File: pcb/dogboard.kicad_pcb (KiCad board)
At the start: 6 copper layers, 50 x 30 mm, 55 parts, among them J1 USB-C / USB2.0, J2 Lights, J3 Current Conn, SW1 BOOT, SW2 Action, SW3 Action, U1 RP2040, U2 L9110H, U3 4MB Flash, U4 BCR430, Y1 12 MHz

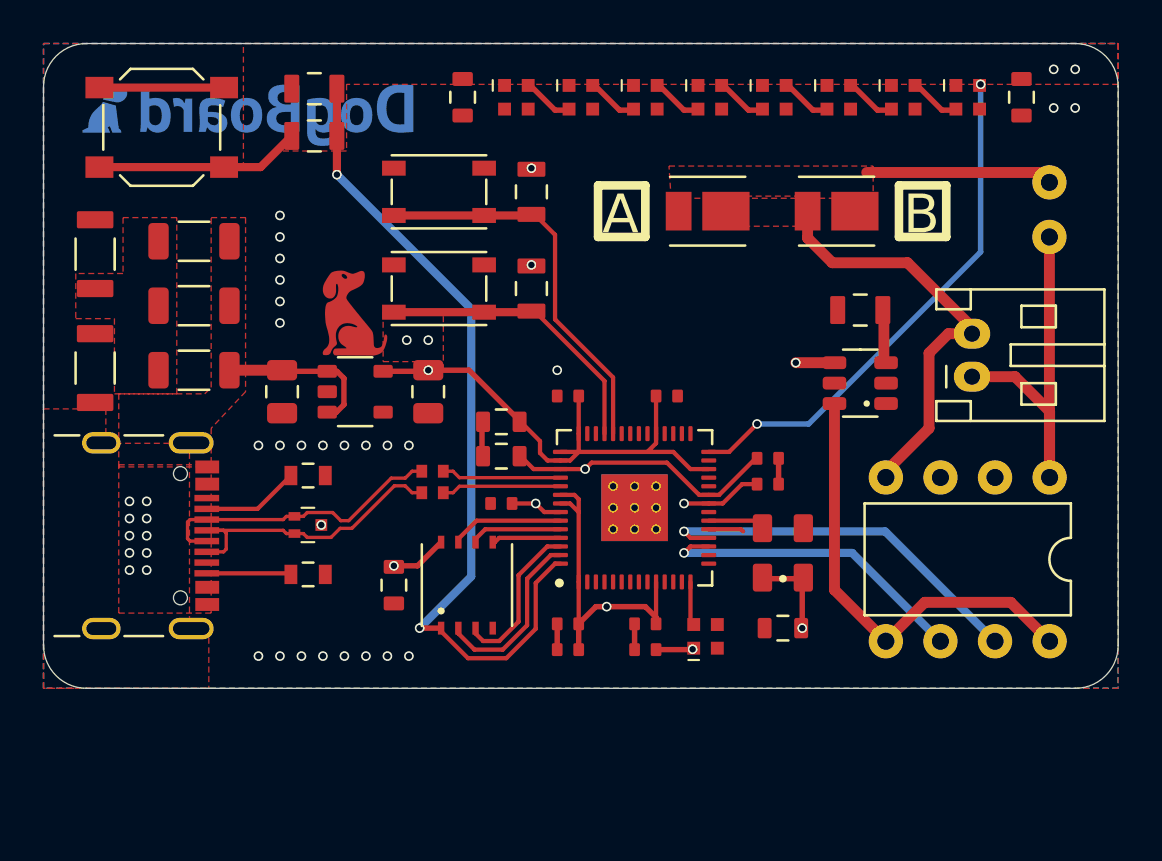
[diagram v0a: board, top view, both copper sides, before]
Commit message: dogboard-2b3
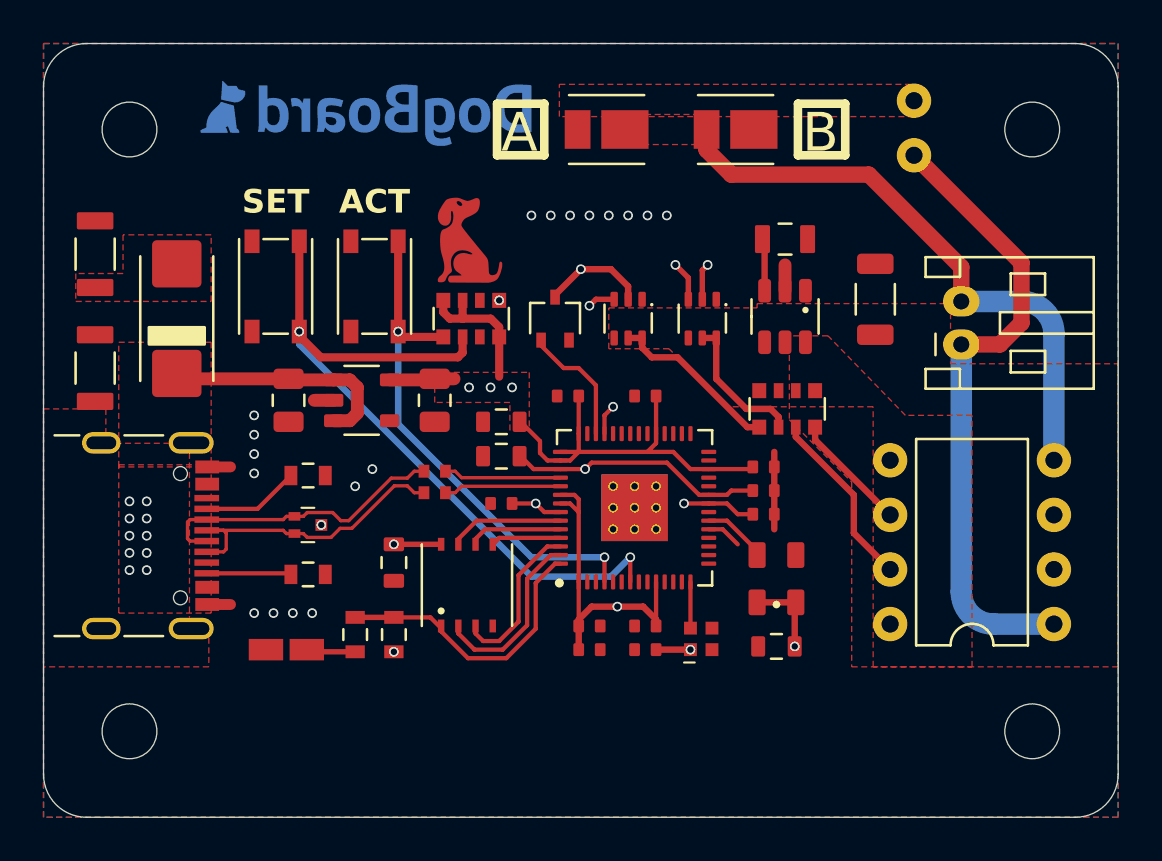
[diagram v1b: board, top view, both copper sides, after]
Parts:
- removed C19, C20: 1uF, _custom:CAP_0603_HandSolder
- removed D10, D2, D3, D4, D5, D7, D8, D9: LED_NeoPixel, _custom:LED_NeoPixel_0606
- removed R12: 10k, _custom:R_0805_HandSolder
- removed SW1: BOOT, _custom:button_metal_smd
- added H1: MountingHole, _custom:MountingHole_M2.5, F.Cu at (128.0, 88.0)
- added H2: MountingHole, _custom:MountingHole_M2.5, F.Cu at (170.0, 88.0)
- added H3: MountingHole, _custom:MountingHole_M2.5, F.Cu at (170.0, 116.0)
- added H4: MountingHole, _custom:MountingHole_M2.5, F.Cu at (128.0, 116.0)
- added JP1: Boot-Jumper, _custom:Jumper_Open_SMD_3.5mm, F.Cu at (135.3, 112.2)
- added Q1: MOSFET, _custom:GenericIC_SOT-363, F.Cu at (154.7, 96.8)
- added Q2: MOSFET, _custom:GenericIC_SOT-363, F.Cu at (151.2, 96.8)
- added Q3: N-MOS, _custom:Transistor_SOT-323, F.Cu at (147.8, 96.8)
- added R9: 10k, _custom:R_Array_4x1206_Convex, F.Cu at (158.6, 101.0)
- C1: value 10uF -> 150uF; footprint _custom:CAP_1206_NoKeepout -> _custom:CAP_Tantalum_2312
- C2: value 10uF -> 10u
- C3: value 10uF -> 0.1u; footprint _custom:CAP_1206_NoKeepout -> _custom:CAP_0402_HandSolder
- R10: footprint _custom:R_0805_HandSolder -> _custom:R_Array_4x1206_Convex
- R4, R6: footprint _custom:R_0805_HandSolder -> _custom:R_0603_HandSolder
- U3: value 4MB Flash -> 8MB Flash
- moved C2 31.7 mm to (162.7, 95.9), turned to 90 degrees
- moved C3 28.5 mm to (157.5, 103.7), turned to 0 degrees
- moved R4 25.7 mm to (140.3, 111.5), turned to -90 degrees
- moved R6 23.3 mm to (138.5, 111.5), turned to -90 degrees
- moved SW3 7.60 mm to (134.8, 95.3), turned to -90 degrees
- moved J3 7.36 mm to (164.5, 89.2)
- moved R10 6.53 mm to (143.9, 96.8)
- moved D12 6.04 mm to (150.2, 88.0)
- moved D13 6.04 mm to (156.2, 88.0)
- moved SW2 5.33 mm to (139.4, 95.3), turned to -90 degrees
- moved R11 4.81 mm to (158.5, 93.1), turned to 0 degrees
- moved U4 4.68 mm to (158.5, 96.7), turned to -90 degrees
- moved C1 2.53 mm to (130.2, 96.8), turned to 90 degrees
- moved J2 1.58 mm to (168.5, 97.0)
- moved C8 1.51 mm to (157.5, 104.8)
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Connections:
- net /OUT_{A} renamed /Output/OUT_{A}
- net /OUT_{B} renamed /Output/OUT_{B}
- net /OUT_{C} renamed /Output/OUT_{C}
- C2 pad 2: /GND_RET -> GNDREF
- C3 pad 1: VBUS -> +3.3V
- C3 pad 2: /GND_RET -> GNDREF
- R6 pad 1: Net-(R6-Pad1) -> /~{BOOT}
- R6 pad 2: /~{BOOT} -> Net-(JP1-A)
- U1 pad 17: /SIG_{A} -> GPIO14
- U1 pad 18: /SIG_{B} -> GPIO15
- U1 pad 38: /BTN_{ACT} -> GPIO26
- U1 pad 39: /BTN_{SET} -> SIG_{A}
- U1 pad 4: GPIO2 -> /BTN_{ACT}
- U1 pad 40: GPIO28 -> SIG_{B}
- U1 pad 7: GPIO5 -> /BTN_{SET}
- U2 pad 6: /SIG_{A} -> /Output/LVL_{A}
- U2 pad 7: /SIG_{B} -> /Output/LVL_{B}
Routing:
- net /Output/LVL_{B}: track 0.00 -> 28.8 mm, vias 0 -> 1
- net /~{BOOT}: track 39.0 -> 13.5 mm, vias 2 -> 0
- net /Output/LVL_{A}: track 0.00 -> 24.8 mm, vias 0 -> 1
- net GPIO17: track 24.3 -> 0.00 mm, vias 2 -> 0
- net /BTN_{SET}: track 13.6 -> 35.2 mm, vias 0 -> 2
- net V_{SS}: track 21.2 -> 0.00 mm
- net /SIG_{B}: track 17.9 -> 0.00 mm, vias 1 -> 0
- net /SIG_{A}: track 14.9 -> 0.00 mm, vias 1 -> 0
- net SIG_{A}: track 0.00 -> 11.5 mm, vias 0 -> 2
- net /Output/OUT_{A}: track 18.6 -> 29.7 mm
- net Net-(R6-Pad1): track 9.55 -> 0.00 mm
- net Net-(Q2A-G_{A}): track 0.00 -> 9.33 mm, vias 0 -> 2
- net /Output/OUT_{C}: track 8.69 -> 0.00 mm
- net Net-(Q2A-D_{A}): track 0.00 -> 8.08 mm
- net /Output/OUT_{B}: track 19.9 -> 27.7 mm
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- added copper zone on F.Cu, net V_{SS}
- removed copper zone on B.Cu, net +3.3V
- removed copper zone on In4.Cu, net +3.3V
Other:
- board size 50 x 30 mm -> 50 x 36 mm
- board text added: "2.0 BETA 3"
- board text added: "ACT"
- board text added: "SET"
- board text removed: "2.0 BETA 2"
